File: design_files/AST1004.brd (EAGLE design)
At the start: 10 x 10 mm, 12 parts, among them J1 SM05B, U1 TCS34725FN

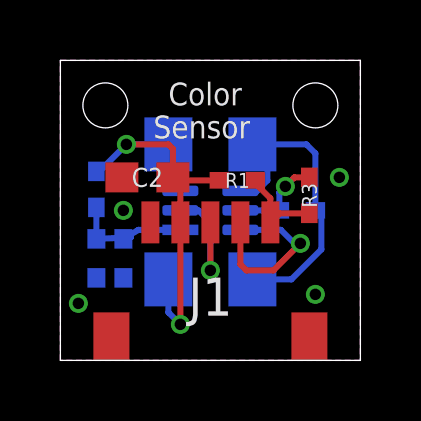
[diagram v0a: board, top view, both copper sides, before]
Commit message: updated documentation
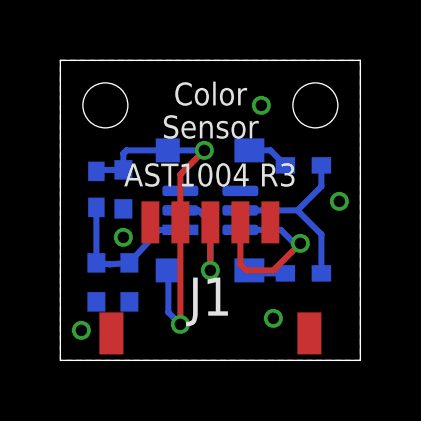
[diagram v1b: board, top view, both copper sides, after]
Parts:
- removed C4: 1uF, tinycircuits:C0402
- removed R4: 5.0, tinycircuits:0402
- added C3: 0.1uF, tinycircuits:C0402
- C1: value 0.1uF -> 1uF
- C2: value 10uF -> 1uF; device tinycircuits:C0603 -> tinycircuits:C0402
- D1, D2: value LED -> QBLP674-IWM-NW; device tinycircuits:C1206 -> tinycircuits:LED_TOP_2.8X1.4
- J1: device tinycircuits:JST_SH_5X1 -> tinycircuits:JST_SH_5X1_EDGE
- R1: value 10.0K -> 27.0
- R2: value 27.0 -> 5K
- R3: value 0.0 -> 5K
- moved R2 6.95 mm to (23.1, 16.5), turned to 0 degrees
- moved R1 4.71 mm to (16.2, 15.7), flipped to the bottom, turned to 270 degrees
- moved C2 3.89 mm to (16.2, 12.6), flipped to the bottom, turned to 270 degrees
- moved R3 2.61 mm to (23.1, 12.9), flipped to the bottom, turned to 0 degrees
- moved C1 2.30 mm to (17.1, 15.7)
- moved D2 0.30 mm to (20.0, 13.0), turned to 0 degrees
- moved D1 0.20 mm to (20.0, 17.0), turned to 0 degrees
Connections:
- removed net LDR: D1.2, D2.2, R4.2, U1.4
- new net N$3: D2.C, R3.2
- new net N$4: D1.C, R2.2
- net GND: now also C3.2; no longer C4.2
- net INT: no longer R1.1, R3.2
- net N$1: now also R2.1; no longer R4.1
- net N$2: now also C2.1, C3.1, R1.2; no longer C1.1, C4.1, R2.2
- net VCC: now also C1.1, D1.A, D2.A, R1.1; no longer C2.1, D1.1, D2.1, R1.2, R2.1
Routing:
- net LDR: track 10.5 -> 0.00 mm
- net N$1: track 3.11 -> 6.16 mm, vias 1 -> 0
- net INT: track 3.03 -> 0.00 mm
- net N$4: track 0.00 -> 1.41 mm
- net N$3: track 0.00 -> 1.24 mm
- net VCC: track 13.6 -> 12.4 mm
- net N$2: track 4.44 -> 5.14 mm
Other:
- board text added: "3"
- board text added: "AST1004 R3"
- board text added: "Wireling Color Sensor"
- board text removed: "2"
- board text removed: "AST1004 R2"
- board text removed: "Color Sensor Board"
